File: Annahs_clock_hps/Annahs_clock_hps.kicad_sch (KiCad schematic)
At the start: 9 parts

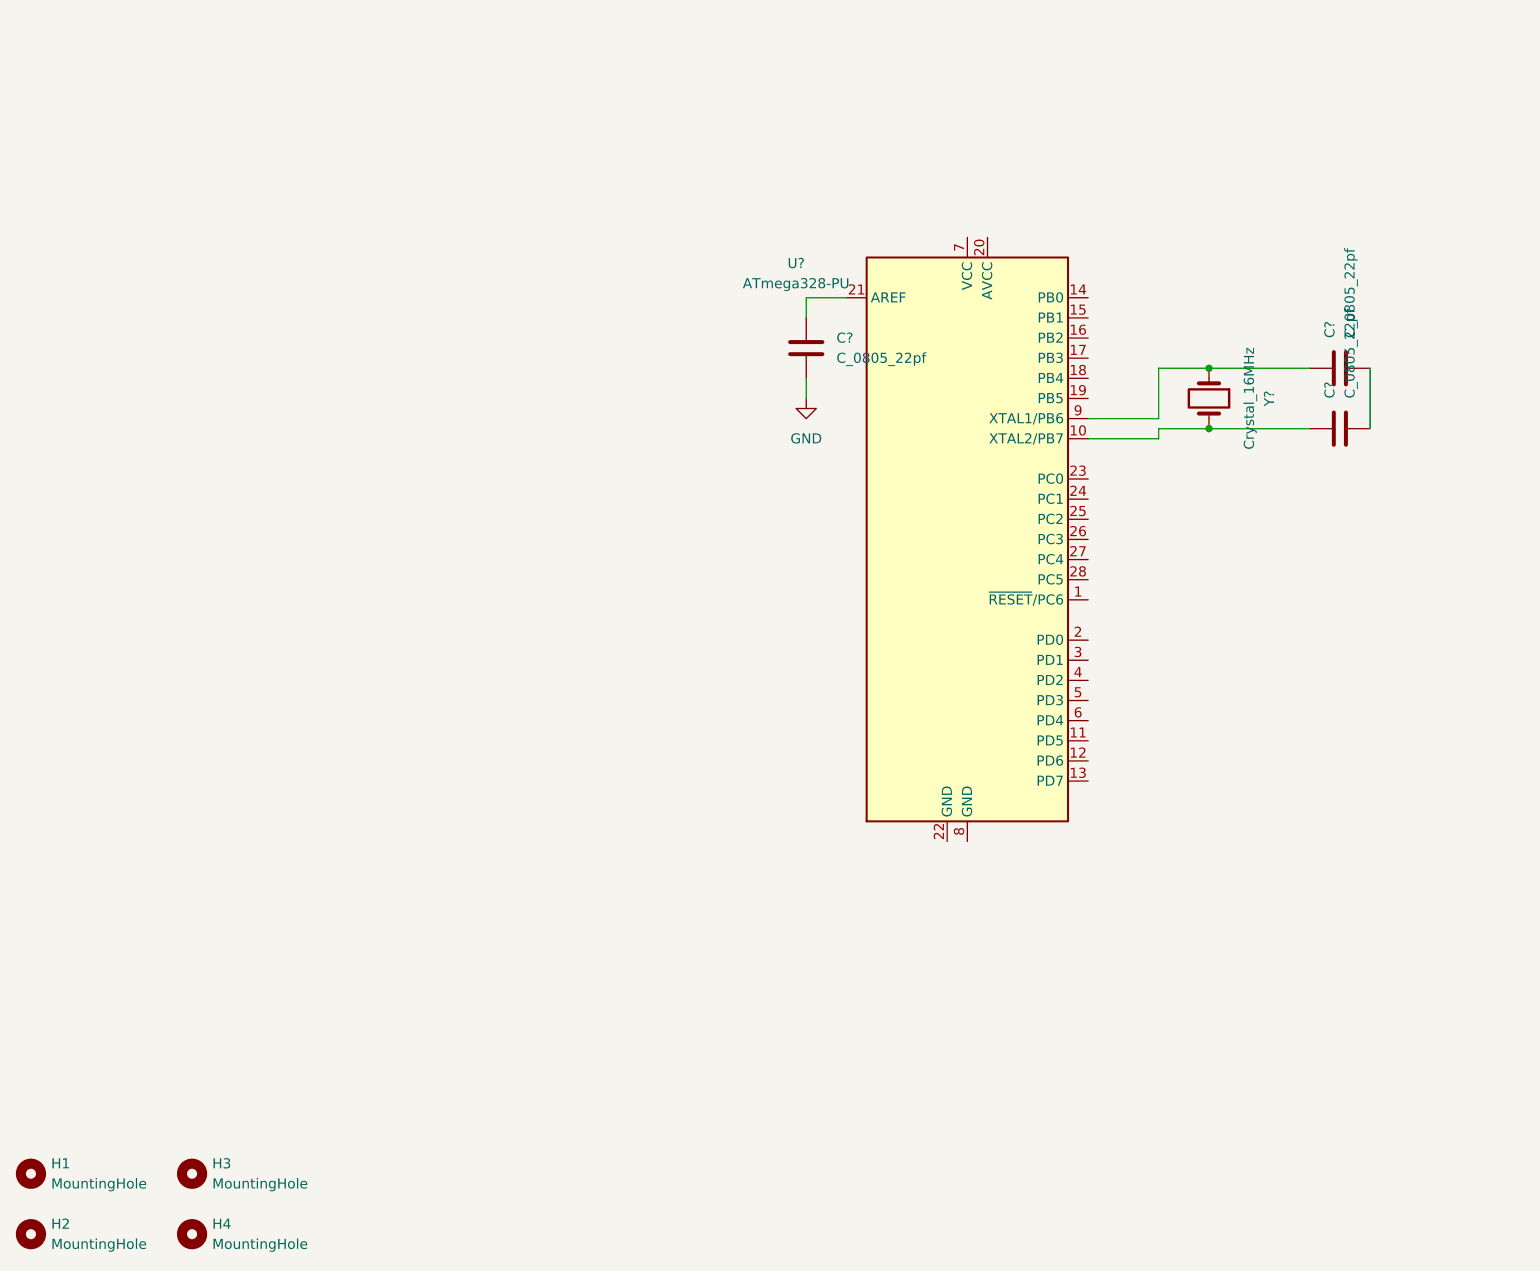
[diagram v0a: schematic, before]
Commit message: Slide 39
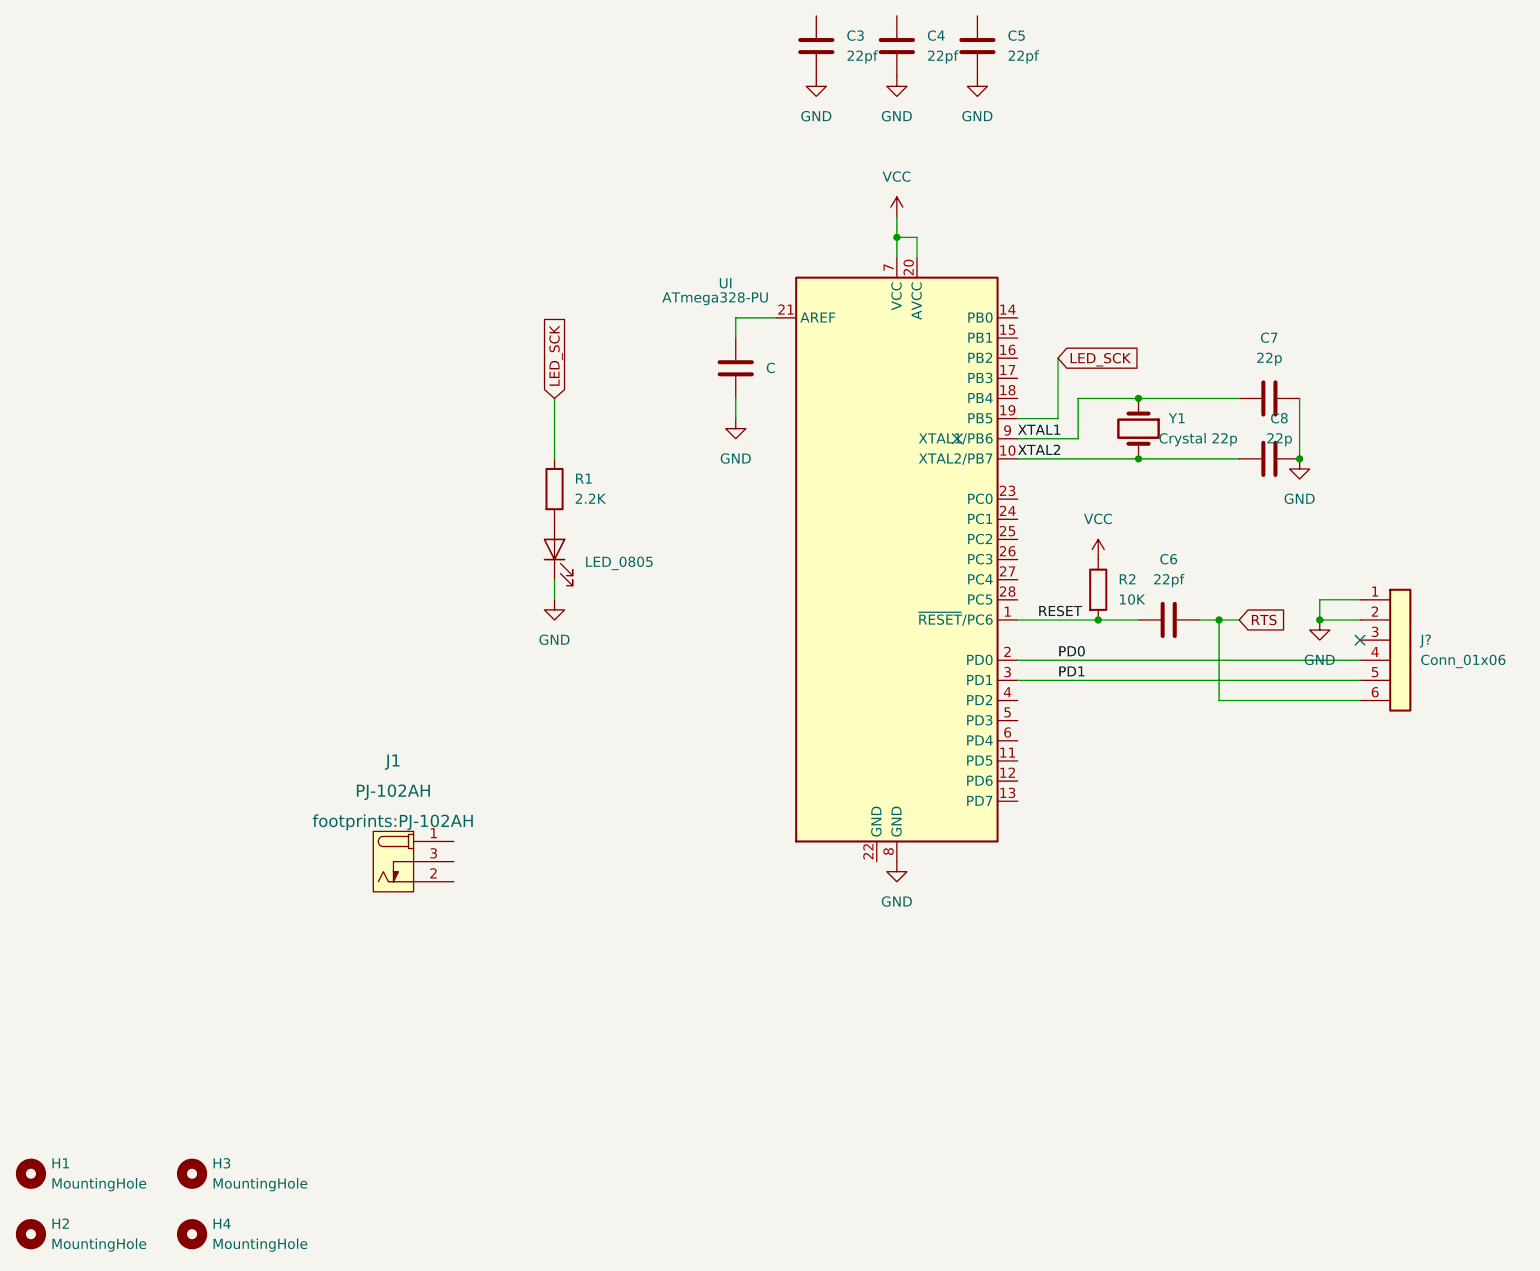
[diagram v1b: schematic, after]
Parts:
- added C3, C4, C5, C6: 22pf, footprints:C_0805_2012Metric, symbol HPS:C_0805_22pf
- added D?: LED_0805, footprints:LED_0805_2012Metric, symbol HPS:LED_0805
- added J1: PJ-102AH, footprints:PJ-102AH, symbol HPS:PJ-102AH
- added J?: Conn_01x06, footprints:PinHeader_1x06_P2.54mm_Vertical, symbol HPS:Conn_01x06
- added R1: 2.2K, footprints:R_0805_2012Metric, symbol HPS:R_0805_2.2K
- added R2: 10K, footprints:R_0805_2012Metric, symbol HPS:R_0805_10K
- C7, C8: renamed from C?; value C_0805_22pf -> 22p
- Y1: renamed from Y?; value Crystal_16MHz -> Crystal 22p
- gave numbers to parts that had none: 2
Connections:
- net GND: now also C7.2, C8.2, UI.8 (GND), C3.2, C4.2, C5.2, D?.1 (K), J?.1 (Pin_1), J?.2 (Pin_2)
- net XTAL1: now reaches C7.1, UI.9 (XTAL1/PB6), Y1.1
- net XTAL2: now reaches C8.1, UI.10 (XTAL2/PB7), Y1.2
- net RESET: now reaches UI.1 (~{RESET}/PC6)
- net RESET: now also C6.2, R2.2
- net LED_SCK: now reaches UI.19 (PB5)
- net LED_SCK: now also R1.1
- net PD0: now reaches UI.2 (PD0)
- net PD0: now also J?.4 (Pin_4)
- net VCC: now reaches UI.20 (AVCC)
- net VCC: now also UI.7 (VCC), R2.1
- net PD1: now reaches UI.3 (PD1)
- net PD1: now also J?.5 (Pin_5)
- new net: D?.2 (A), R1.2
- new net RTS: C6.1, J?.6 (Pin_6)
- no-connect marks 0 -> 2
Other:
- moved on the sheet: C, C7, C8, UI, Y1
